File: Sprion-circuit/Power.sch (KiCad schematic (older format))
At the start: 27 parts, among them IC1 R3111N211A, IC2 TAR5SB50, J1 Conn_01x02_Female, Q1 Q_PMOS_GSD, Q2 Q_NMOS_GSD, SW1 SW_SPDT, U4 LXDC55FAAA-203

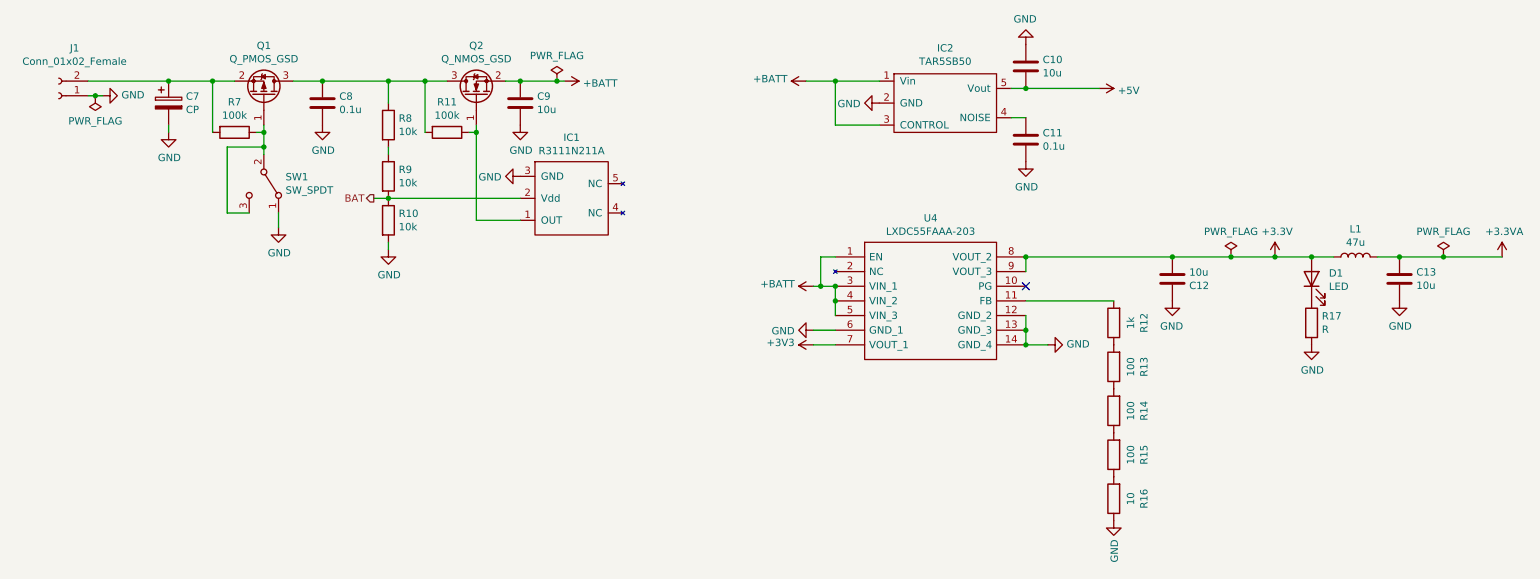
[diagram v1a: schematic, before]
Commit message: :fix　いろいろ
後で書きます
とりあえず寝ます
許してください
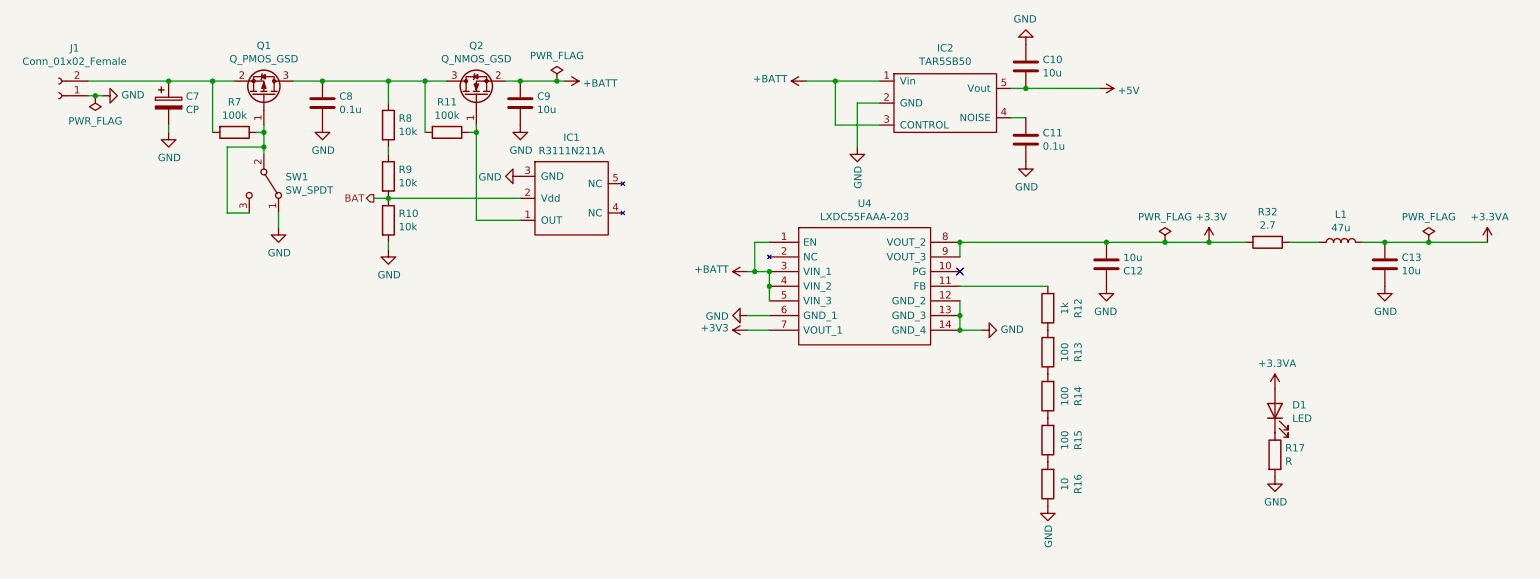
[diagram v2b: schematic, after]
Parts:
- added R32: 2.7, symbol Device:R
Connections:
- net +3.3VA: now also D1.2 (A)
- net +3V3: now also R32.2; no longer D1.2 (A), L1.1
- new net: L1.1, R32.1
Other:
- moved on the sheet: C12, C13, D1, L1, R12, R13, R14, R15, R16, R17, U4
